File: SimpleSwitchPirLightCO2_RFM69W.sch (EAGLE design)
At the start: 57 parts, among them IC3 MC33269ST-3.3T3, K1 FRS1B, K2 FRS1B, K3 FRS1B, Q1 BC327SMD, T1 BC846, T2 BC846, T3 BC846, T4 BC846, X1 16 MHz

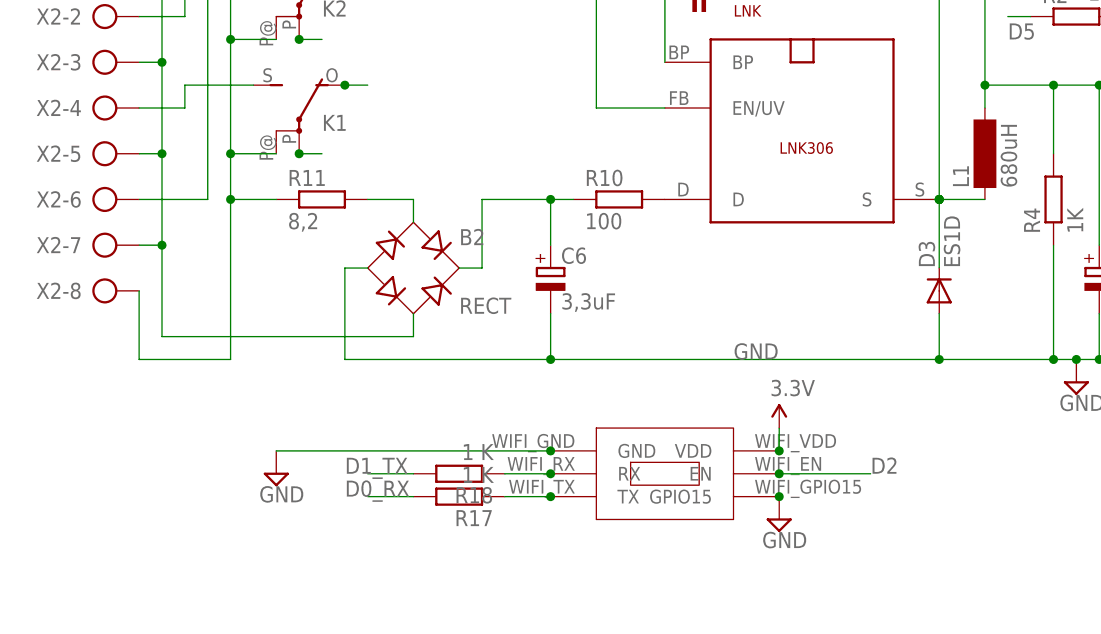
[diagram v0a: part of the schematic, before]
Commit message: bugfix
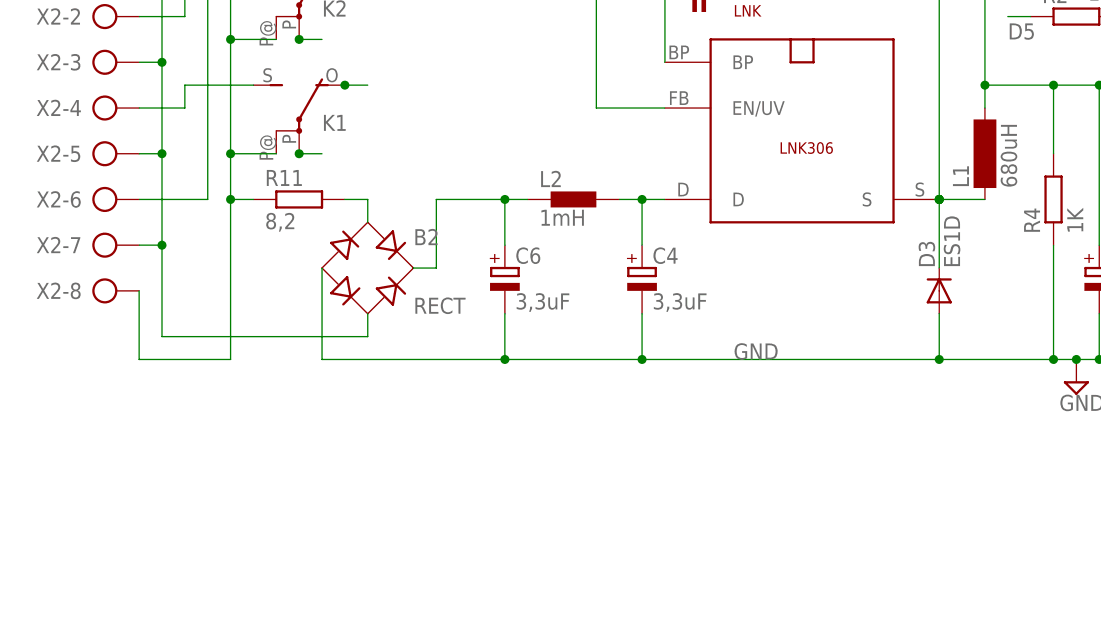
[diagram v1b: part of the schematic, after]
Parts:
- removed R10: 100, resistor:R-EU_R2512W
- removed R17, R18: 1 K, resistor:R-EU_M2012
- removed U$5: ESP03, RemoteHome:ESP03
- added C4: 3,3uF, resistor:CPOL-EUE5-10.5
- added L2: 1mH, inductors:BL02RN1
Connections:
- removed net N$28: R17.1, U$5.TX
- removed net N$29: R18.1, U$5.RX
- net D0_RX: no longer R17.2
- net D1_TX: no longer R18.2
- net D2: no longer U$5.EN
- net GND: now also C4.-; no longer U$5.GND, U$5.GPIO15
- net N$13: now also C4.+, L2.2; no longer R10.2
- net N$14: now also L2.1; no longer R10.1
- net VCC: no longer U$5.VDD
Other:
- moved on the sheet: B2, C6, R11
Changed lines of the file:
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@@
 <part name="LNK" library="powerint" deviceset="SO-8C" device="" value="LNK306"/>
 <part name="B2" library="rectifier" deviceset="RECTIFIER-" device="S40" value="RECT"/>
-<part name="R10" library="resistor" deviceset="R-EU_" device="R2512W" value="100"/>
 <part name="R11" library="resistor" deviceset="R-EU_" device="0411/12" value="8,2"/>
 <part name="C6" library="resistor" deviceset="CPOL-EU" device="E5-10.5" value="3,3uF"/>
@@
 <part name="X2" library="con-ptr500" deviceset="AK500/8" device=""/>
 <part name="R14" library="resistor" deviceset="R-EU_" device="M2012" value="1 K"/>
-<part name="SUPPLY16" library="supply2" deviceset="GND" device=""/>
-<part name="SUPPLY17" library="SparkFun" deviceset="VCC" device="" value="3.3V"/>
-<part name="R17" library="resistor" deviceset="R-EU_" device="M2012" value="1 K"/>
-<part name="R18" library="resistor" deviceset="R-EU_" device="M2012" value="1 K"/>
-<part name="U$5" library="RemoteHome" deviceset="ESP03" device=""/>
-<part name="SUPPLY18" library="supply2" deviceset="GND" device=""/>
+<part name="L2" library="inductors" deviceset="BL0" device="2RN1" value="1mH"/>
+<part name="C4" library="resistor" deviceset="CPOL-EU" device="E5-10.5" value="3,3uF"/>
 </parts>
 <sheets>
@@
 <attribute name="VALUE" x="93.98" y="55.88" size="1.27" layer="94"/>
 </instance>
-<instance part="B2" gate="G$1" x="53.34" y="43.18"/>
-<instance part="R10" gate="G$1" x="76.2" y="50.8"/>
-<instance part="R11" gate="G$1" x="43.18" y="50.8"/>
-<instance part="C6" gate="G$1" x="68.58" y="43.18"/>
+<instance part="B2" gate="G$1" x="48.26" y="43.18"/>
+<instance part="R11" gate="G$1" x="40.64" y="50.8"/>
+<instance part="C6" gate="G$1" x="63.5" y="43.18"/>
 <instance part="C7" gate="G$1" x="83.82" y="73.66" rot="R90"/>
 <instance part="R12" gate="G$1" x="86.36" y="83.82" rot="R180"/>
@@
 <attribute name="VALUE" x="161.29" y="67.818" size="1.778" layer="96"/>
 </instance>
-<instance part="SUPPLY16" gate="GND" x="38.1" y="20.32"/>
-<instance part="SUPPLY17" gate="1" x="93.98" y="25.4"/>
-<instance part="R17" gate="G$1" x="58.42" y="17.78" rot="R180"/>
-<instance part="R18" gate="G$1" x="58.42" y="20.32" rot="R180"/>
-<instance part="U$5" gate="G$1" x="76.2" y="20.32"/>
-<instance part="SUPPLY18" gate="GND" x="93.98" y="15.24"/>
+<instance part="L2" gate="G$1" x="71.12" y="50.8"/>
+<instance part="C4" gate="G$1" x="78.74" y="43.18"/>
 </instances>
 <busses>
@@
 <pinref part="T1" gate="G$1" pin="E"/>
 <pinref part="B2" gate="G$1" pin="-"/>
-<wire x1="48.26" y1="43.18" x2="45.72" y2="43.18" width="0.1524" layer="91"/>
-<wire x1="45.72" y1="43.18" x2="45.72" y2="33.02" width="0.1524" layer="91"/>
-<wire x1="45.72" y1="33.02" x2="68.58" y2="33.02" width="0.1524" layer="91"/>
-<wire x1="68.58" y1="33.02" x2="111.76" y2="33.02" width="0.1524" layer="91"/>
+<wire x1="43.18" y1="43.18" x2="43.18" y2="33.02" width="0.1524" layer="91"/>
+<wire x1="43.18" y1="33.02" x2="63.5" y2="33.02" width="0.1524" layer="91"/>
+<wire x1="63.5" y1="33.02" x2="78.74" y2="33.02" width="0.1524" layer="91"/>
+<wire x1="78.74" y1="33.02" x2="111.76" y2="33.02" width="0.1524" layer="91"/>
 <wire x1="111.76" y1="33.02" x2="124.46" y2="33.02" width="0.1524" layer="91"/>
 <wire x1="124.46" y1="33.02" x2="127" y2="33.02" width="0.1524" layer="91"/>
@@
 <junction x="167.64" y="33.02"/>
 <pinref part="C6" gate="G$1" pin="-"/>
-<wire x1="68.58" y1="38.1" x2="68.58" y2="33.02" width="0.1524" layer="91"/>
-<junction x="68.58" y="33.02"/>
+<wire x1="63.5" y1="38.1" x2="63.5" y2="33.02" width="0.1524" layer="91"/>
+<junction x="63.5" y="33.02"/>
 <junction x="127" y="33.02"/>
 <pinref part="D3" gate="G$1" pin="A"/>
@@
 <wire x1="170.18" y1="66.04" x2="152.4" y2="66.04" width="0.1524" layer="91"/>
 <junction x="152.4" y="66.04"/>
+<pinref part="C4" gate="G$1" pin="-"/>
+<wire x1="78.74" y1="38.1" x2="78.74" y2="33.02" width="0.1524" layer="91"/>
+<junction x="78.74" y="33.02"/>
 </segment>
 <segment>
@@
 <pinref part="SUPPLY12" gate="GND" pin="GND"/>
 </segment>
-<segment>
-<pinref part="U$5" gate="G$1" pin="GND"/>
-<wire x1="68.58" y1="22.86" x2="38.1" y2="22.86" width="0.1524" layer="91"/>
-<pinref part="SUPPLY16" gate="GND" pin="GND"/>
-<junction x="68.58" y="22.86"/>
-</segment>
-<segment>
-<pinref part="U$5" gate="G$1" pin="GPIO15"/>
-<pinref part="SUPPLY18" gate="GND" pin="GND"/>
-<junction x="93.98" y="17.78"/>
-</segment>
 </net>
 <net name="D10_SS" class="0">
@@
 <wire x1="81.28" y1="165.1" x2="88.9" y2="165.1" width="0.1524" layer="91"/>
 </segment>
-<segment>
-<wire x1="93.98" y1="22.86" x2="93.98" y2="25.4" width="0.1524" layer="91"/>
-<pinref part="SUPPLY17" gate="1" pin="VCC"/>
-<pinref part="U$5" gate="G$1" pin="VDD"/>
-<junction x="93.98" y="22.86"/>
-</segment>
 </net>
 <net name="D9" class="0">
@@
 <pinref part="INTERFACE" gate="G$1" pin="4"/>
 </segment>
-<segment>
-<pinref part="R18" gate="G$1" pin="2"/>
-<wire x1="53.34" y1="20.32" x2="48.26" y2="20.32" width="0.1524" layer="91"/>
-<label x="45.72" y="20.32" size="1.778" layer="95"/>
-</segment>
 </net>
 <net name="D0_RX" class="0">
@@
 <wire x1="68.58" y1="132.08" x2="100.33" y2="132.08" width="0.1524" layer="91"/>
 <pinref part="INTERFACE" gate="G$1" pin="3"/>
-</segment>
-<segment>
-<pinref part="R17" gate="G$1" pin="2"/>
-<wire x1="53.34" y1="17.78" x2="48.26" y2="17.78" width="0.1524" layer="91"/>
-<label x="45.72" y="17.78" size="1.778" layer="95"/>
 </segment>
 </net>
@@
 <label x="116.84" y="127" size="1.778" layer="95"/>
 </segment>
-<segment>
-<wire x1="93.98" y1="20.32" x2="104.14" y2="20.32" width="0.1524" layer="91"/>
-<label x="104.14" y="20.32" size="1.778" layer="95"/>
-<pinref part="U$5" gate="G$1" pin="EN"/>
-<junction x="93.98" y="20.32"/>
-</segment>
 </net>
 <net name="D11_MOSI" class="0">
@@
 </segment>
 </net>
-<net name="N$3" class="0">
-<segment>
-<pinref part="U$1" gate="G$1" pin="1"/>
-<wire x1="160.02" y1="127" x2="157.48" y2="127" width="0.1524" layer="91"/>
-<pinref part="RFM69" gate="G$1" pin="ANT"/>
-</segment>
-</net>
 <net name="N$8" class="2">
 <segment>
 <pinref part="R11" gate="G$1" pin="1"/>
-<wire x1="33.02" y1="50.8" x2="38.1" y2="50.8" width="0.1524" layer="91"/>
+<wire x1="33.02" y1="50.8" x2="35.56" y2="50.8" width="0.1524" layer="91"/>
 <junction x="33.02" y="50.8"/>
 <wire x1="33.02" y1="50.8" x2="33.02" y2="33.02" width="0.1524" layer="91"/>
@@
 <segment>
 <pinref part="B2" gate="G$1" pin="AC2"/>
-<wire x1="53.34" y1="38.1" x2="53.34" y2="35.56" width="0.1524" layer="91"/>
-<wire x1="53.34" y1="35.56" x2="25.4" y2="35.56" width="0.1524" layer="91"/>
+<wire x1="48.26" y1="38.1" x2="48.26" y2="35.56" width="0.1524" layer="91"/>
+<wire x1="48.26" y1="35.56" x2="25.4" y2="35.56" width="0.1524" layer="91"/>
 <wire x1="25.4" y1="45.72" x2="25.4" y2="35.56" width="0.1524" layer="91"/>
 <wire x1="25.4" y1="45.72" x2="25.4" y2="55.88" width="0.1524" layer="91"/>
@@
 </segment>
 </net>
-<net name="N$13" class="2">
-<segment>
-<pinref part="LNK" gate="G$1" pin="D"/>
-<pinref part="R10" gate="G$1" pin="2"/>
-</segment>
-</net>
 <net name="N$14" class="2">
 <segment>
 <pinref part="B2" gate="G$1" pin="+"/>
-<wire x1="58.42" y1="43.18" x2="60.96" y2="43.18" width="0.1524" layer="91"/>
-<wire x1="60.96" y1="43.18" x2="60.96" y2="50.8" width="0.1524" layer="91"/>
-<wire x1="60.96" y1="50.8" x2="68.58" y2="50.8" width="0.1524" layer="91"/>
-<pinref part="R10" gate="G$1" pin="1"/>
+<wire x1="53.34" y1="43.18" x2="55.88" y2="43.18" width="0.1524" layer="91"/>
+<wire x1="55.88" y1="43.18" x2="55.88" y2="50.8" width="0.1524" layer="91"/>
+<wire x1="55.88" y1="50.8" x2="63.5" y2="50.8" width="0.1524" layer="91"/>
+<pinref part="L2" gate="G$1" pin="1"/>
 <pinref part="C6" gate="G$1" pin="+"/>
-<wire x1="68.58" y1="50.8" x2="71.12" y2="50.8" width="0.1524" layer="91"/>
-<wire x1="68.58" y1="45.72" x2="68.58" y2="50.8" width="0.1524" layer="91"/>
-<junction x="68.58" y="50.8"/>
+<wire x1="63.5" y1="50.8" x2="66.04" y2="50.8" width="0.1524" layer="91"/>
+<wire x1="63.5" y1="45.72" x2="63.5" y2="50.8" width="0.1524" layer="91"/>
+<junction x="63.5" y="50.8"/>
 </segment>
 </net>
@@
 <segment>
 <pinref part="R11" gate="G$1" pin="2"/>
-<wire x1="48.26" y1="50.8" x2="53.34" y2="50.8" width="0.1524" layer="91"/>
+<wire x1="45.72" y1="50.8" x2="48.26" y2="50.8" width="0.1524" layer="91"/>
 <pinref part="B2" gate="G$1" pin="AC1"/>
-<wire x1="53.34" y1="50.8" x2="53.34" y2="48.26" width="0.1524" layer="91"/>
+<wire x1="48.26" y1="50.8" x2="48.26" y2="48.26" width="0.1524" layer="91"/>
 </segment>
 </net>
@@
 </segment>
 </net>
-<net name="N$28" class="0">
-<segment>
-<pinref part="R17" gate="G$1" pin="1"/>
-<wire x1="68.58" y1="17.78" x2="63.5" y2="17.78" width="0.1524" layer="91"/>
-<pinref part="U$5" gate="G$1" pin="TX"/>
-<junction x="68.58" y="17.78"/>
-</segment>
-</net>
-<net name="N$29" class="0">
-<segment>
-<wire x1="68.58" y1="20.32" x2="63.5" y2="20.32" width="0.1524" layer="91"/>
-<pinref part="R18" gate="G$1" pin="1"/>
-<pinref part="U$5" gate="G$1" pin="RX"/>
-<junction x="68.58" y="20.32"/>
-</segment>
-</net>
+<net name="N$13" class="2">
+<segment>
+<pinref part="LNK" gate="G$1" pin="D"/>
+<pinref part="L2" gate="G$1" pin="2"/>
+<wire x1="81.28" y1="50.8" x2="78.74" y2="50.8" width="0.1524" layer="91"/>
+<pinref part="C4" gate="G$1" pin="+"/>
+<wire x1="78.74" y1="50.8" x2="76.2" y2="50.8" width="0.1524" layer="91"/>
+<wire x1="78.74" y1="45.72" x2="78.74" y2="50.8" width="0.1524" layer="91"/>
+<junction x="78.74" y="50.8"/>
+</segment>
+</net>
+<net name="N$3" class="0">
+<segment>
+<pinref part="U$1" gate="G$1" pin="1"/>
+<pinref part="RFM69" gate="G$1" pin="ANT"/>
+<wire x1="160.02" y1="127" x2="157.48" y2="127" width="0.1524" layer="91"/>
+</segment>
+</net>
